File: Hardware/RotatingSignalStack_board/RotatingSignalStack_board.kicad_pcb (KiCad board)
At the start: 2 copper layers, 81.3 x 71.1 mm, 30 parts, among them J1 8P8C_LED_Shielded, J2 Conn_01x05_Pin, SW1 SW_Push, SW2 SW_Push, U1 OKI, U3 Teensy4.1_DEV-16771

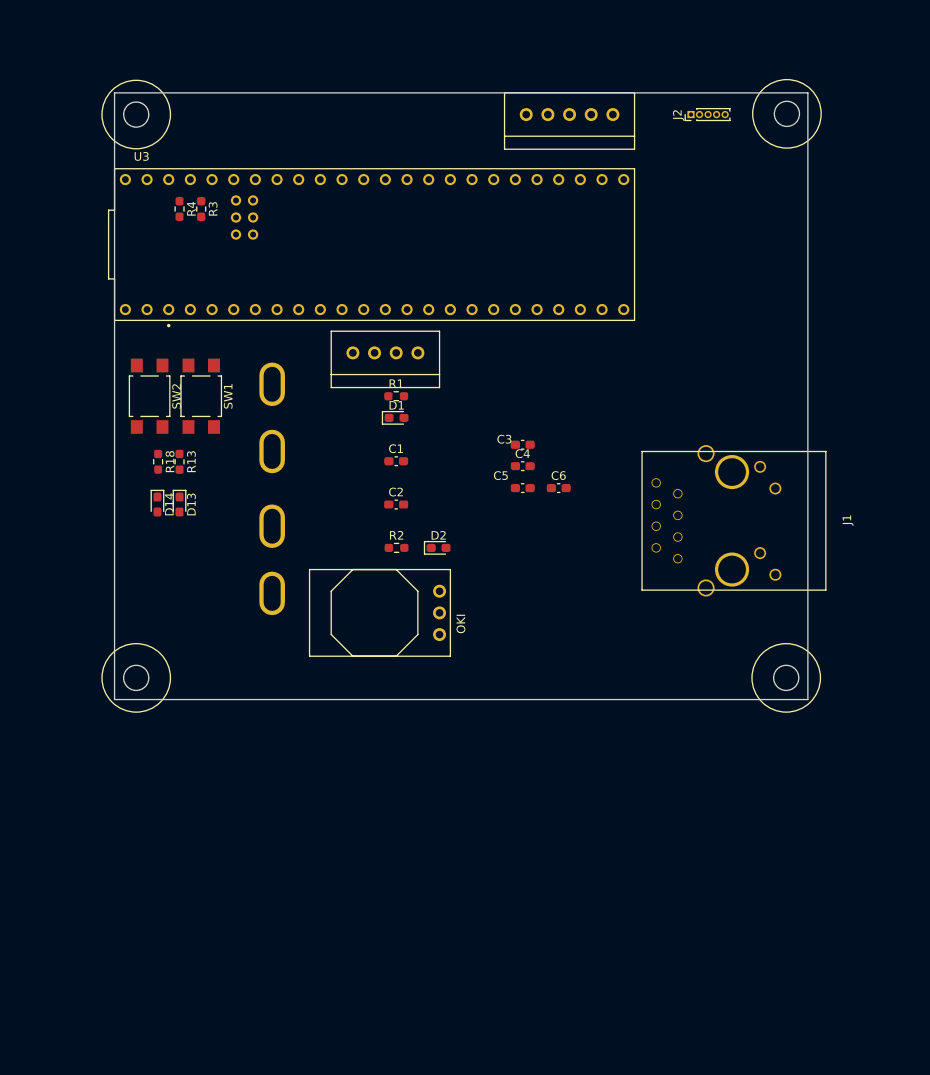
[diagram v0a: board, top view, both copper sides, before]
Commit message: first layout commit - lots of expected changes
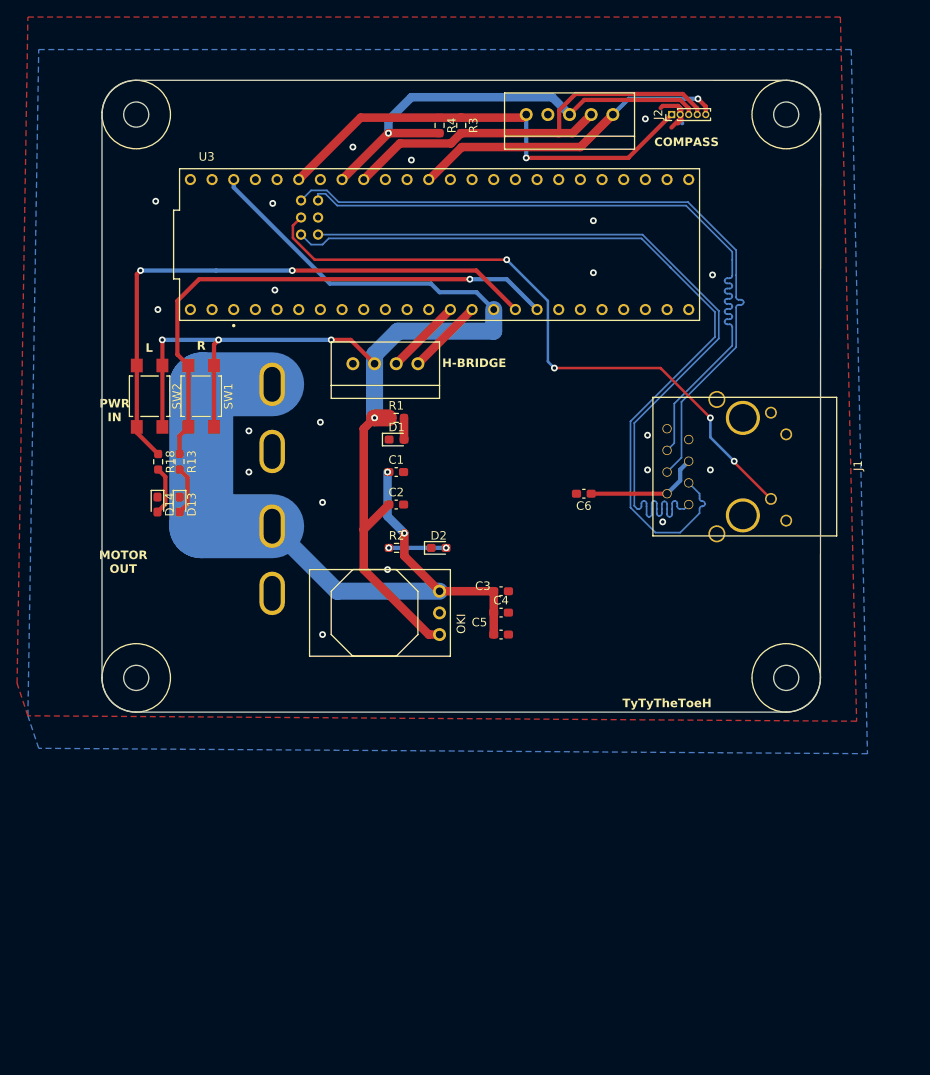
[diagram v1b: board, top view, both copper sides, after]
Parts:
- moved R3 32.0 mm to (144.8, 47.0)
- moved R4 32.0 mm to (142.2, 47.0)
- moved C4 17.4 mm to (149.5, 104.1)
- moved C5 17.4 mm to (149.5, 106.7)
- moved C3 17.4 mm to (149.5, 101.6)
- moved U3 7.62 mm to (142.2, 61.0)
- moved J1 6.48 mm to (190.8, 86.9)
- moved C6 3.02 mm to (159.2, 90.2), turned to 180 degrees
- moved R1 2.54 mm to (137.2, 81.3)
- moved D1 2.54 mm to (137.2, 83.8)
- moved J2 2.27 mm to (169.4, 45.7)
- moved Conn5 1.27 mm to (139.7, 74.9)
- moved C1 1.27 mm to (137.2, 87.6)
- moved V2 0.12 mm to (178.9, 49.7)
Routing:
- net +3.3V: track 0.00 -> 145.2 mm, vias 0 -> 4
- net /Tx-: track 0.00 -> 95.0 mm
- net /Tx+: track 0.00 -> 94.8 mm
- net /Rx+: track 0.00 -> 85.0 mm
- net /Rx-: track 0.00 -> 84.8 mm
- net +12V: track 0.00 -> 83.9 mm, vias 0 -> 2
- net /LED: track 0.00 -> 77.1 mm, vias 0 -> 4
- net JOG B: track 0.00 -> 68.6 mm, vias 0 -> 2
- net JOG A: track 0.00 -> 63.6 mm, vias 0 -> 1
- net I2C SCL: track 0.00 -> 54.2 mm, vias 0 -> 1
- net COMP PWR: track 0.00 -> 54.1 mm, vias 0 -> 1
- net I2C SDA: track 0.00 -> 52.6 mm
- net MAG ENABLE: track 0.00 -> 37.7 mm, vias 0 -> 1
- net Net-(C6-Pad1): track 0.00 -> 13.8 mm
- net GND: track 0.00 -> 9.77 mm, vias 0 -> 20
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- added copper zone on B.Cu, net GND
- added copper zone on F.Cu, net GND
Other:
- board size 81.3 x 71.1 mm -> 84.3 x 74.1 mm
- board text added: "COMPASS"
- board text added: "H-BRIDGE"
- board text added: "L"
- board text added: "MOTOR OUT"
- board text added: "PWR IN"
- board text added: "R"
- board text added: "TyTyTheToeH"

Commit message: changes layout reveiw 1
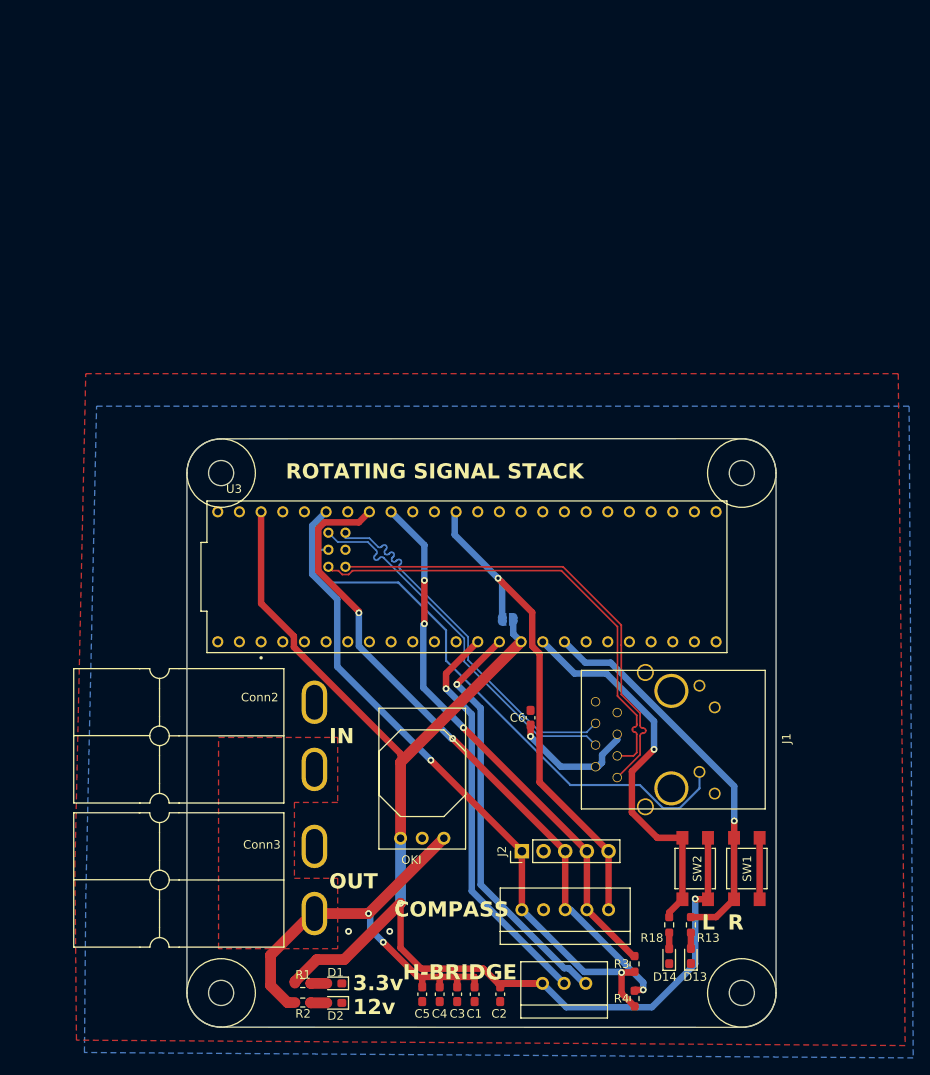
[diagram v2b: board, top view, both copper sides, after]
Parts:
- removed Conn5: Molex_SL_04, MRDT_Connectors:MOLEX_SL_04_Vertical
- added Conn1: Molex_SL_03, MRDT_Connectors:MOLEX_SL_03_Vertical, F.Cu at (159.4, 147.6)
- added R5: 0, Jumper:SolderJumper-2_P1.3mm_Open_RoundedPad1.0x1.5mm, B.Cu at (150.2, 104.9)
- Conn2, Conn3: moved to F.Cu
- J2: footprint Connector_PinHeader_1.00mm:PinHeader_1x05_P1.00mm_Vertical -> Connector_PinHeader_2.54mm:PinHeader_1x05_P2.54mm_Vertical
- moved R4 104.9 mm to (165.1, 149.4), turned to 90 degrees
- moved R3 100.4 mm to (165.1, 145.3), turned to 90 degrees
- moved Conn6 93.2 mm to (162.1, 138.9)
- moved J2 88.1 mm to (151.9, 132.1)
- moved SW1 84.6 mm to (178.3, 134.1)
- moved SW2 84.6 mm to (172.2, 134.1)
- moved R13 80.9 mm to (171.7, 140.7)
- moved R18 80.9 mm to (169.2, 140.7)
- moved D14 80.0 mm to (169.2, 144.4), turned to 90 degrees
- moved D13 80.0 mm to (171.7, 144.4), turned to 90 degrees
- moved V1 75.7 mm to (173.7, 91.8), turned to 0 degrees
- moved V2 71.8 mm to (120.6, 91.8), turned to 90 degrees
- moved R1 67.2 mm to (126.2, 147.5)
- moved D1 64.2 mm to (129.9, 147.6), turned to 180 degrees
- moved C1 61.9 mm to (146.4, 148.8), turned to -90 degrees
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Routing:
- net /Rx+: track 85.0 -> 44.4 mm
- net /Rx-: track 84.8 -> 44.3 mm
- net HB_FWD: track 8.98 -> 48.8 mm, vias 0 -> 1
- net /Tx-: track 95.0 -> 55.8 mm
- net /Tx+: track 94.8 -> 55.8 mm
- net HB_RVS: track 8.98 -> 47.3 mm, vias 0 -> 1
- net +12V: track 83.9 -> 54.4 mm
- net COMP PWR: track 54.1 -> 78.4 mm, vias 1 -> 2
- net I2C SCL: track 54.2 -> 78.2 mm, vias 1 -> 3
- net JOG B: track 68.6 -> 45.8 mm, vias 2 -> 1
- net MAG ENABLE: track 37.7 -> 59.2 mm
- net +3.3V: track 145.2 -> 165.1 mm, vias 4 -> 2
- net JOG A: track 63.6 -> 46.1 mm
- net /LED: track 77.1 -> 64.8 mm, vias 4 -> 0
- net I2C SDA: track 52.6 -> 64.1 mm, vias 0 -> 3
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- added copper zone on F.Cu, net +12V
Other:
- board size 84.3 x 74.1 mm -> 69.1 x 69 mm
- board text added: "12v"
- board text added: "3.3v"
- board text added: "3.3v Direct Pwr Compass"
- board text added: "IN"
- board text added: "OUT"
- board text added: "ROTATING SIGNAL STACK"
- board text removed: "MOTOR OUT"
- board text removed: "PWR IN"
- board text removed: "TyTyTheToeH"
